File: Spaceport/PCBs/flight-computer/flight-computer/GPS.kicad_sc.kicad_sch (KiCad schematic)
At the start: 2 parts, among them U1 SAM-M10Q-00B

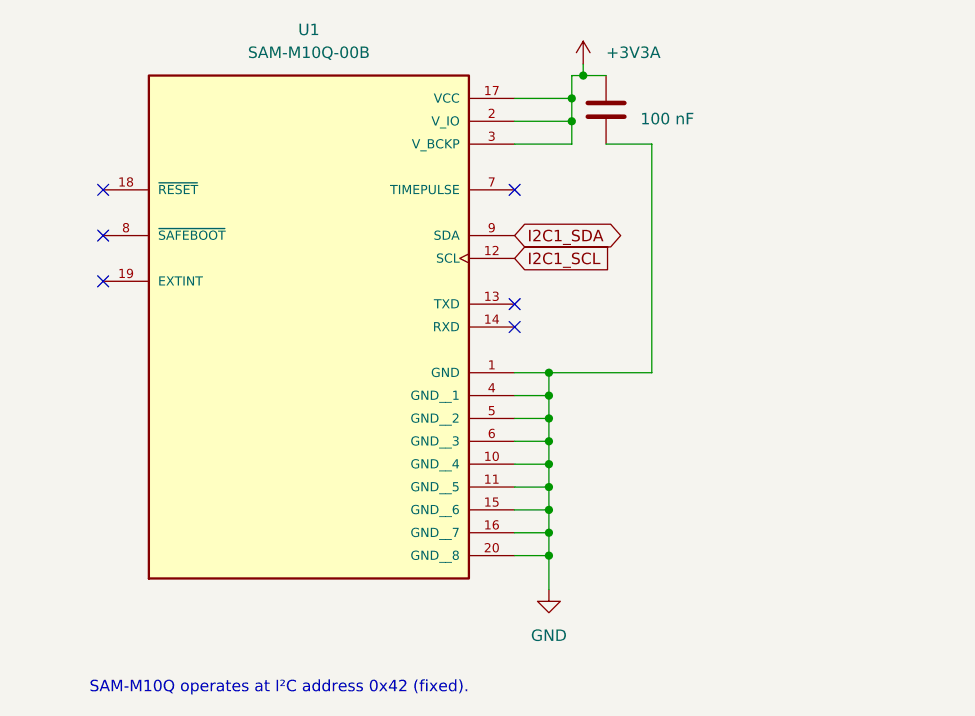
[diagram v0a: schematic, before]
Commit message: removed SdCard
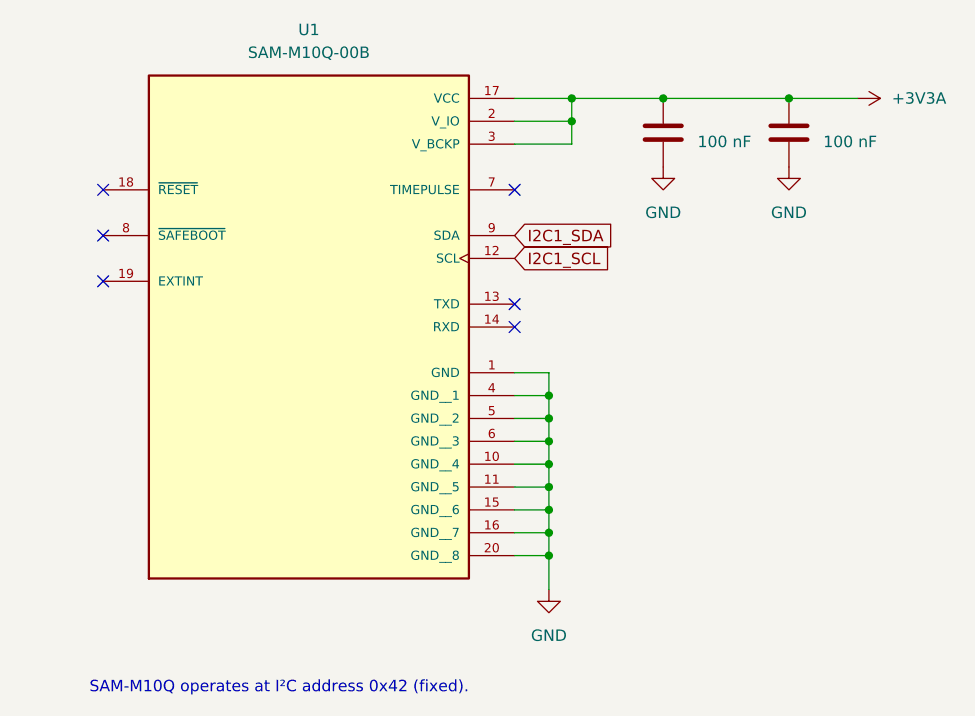
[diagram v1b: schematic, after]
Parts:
- added C18: 100 nF, symbol Device:C
- renumbered C1 to C?
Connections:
- net +3V3A: now also C18.1
- net GND: now also C18.2
